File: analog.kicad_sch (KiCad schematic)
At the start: 36 parts, among them IC6 MCP6S91-E_MS, IC7 MCP6S91-E_MS, IC8 MCP4726A0T-E_CH, K1 AQY210EHAX, K2 AQY210EHAX, U10 MCP6022T-I_SN, U8 MCP6022T-I_SN, U9 MCP6022T-I_SN

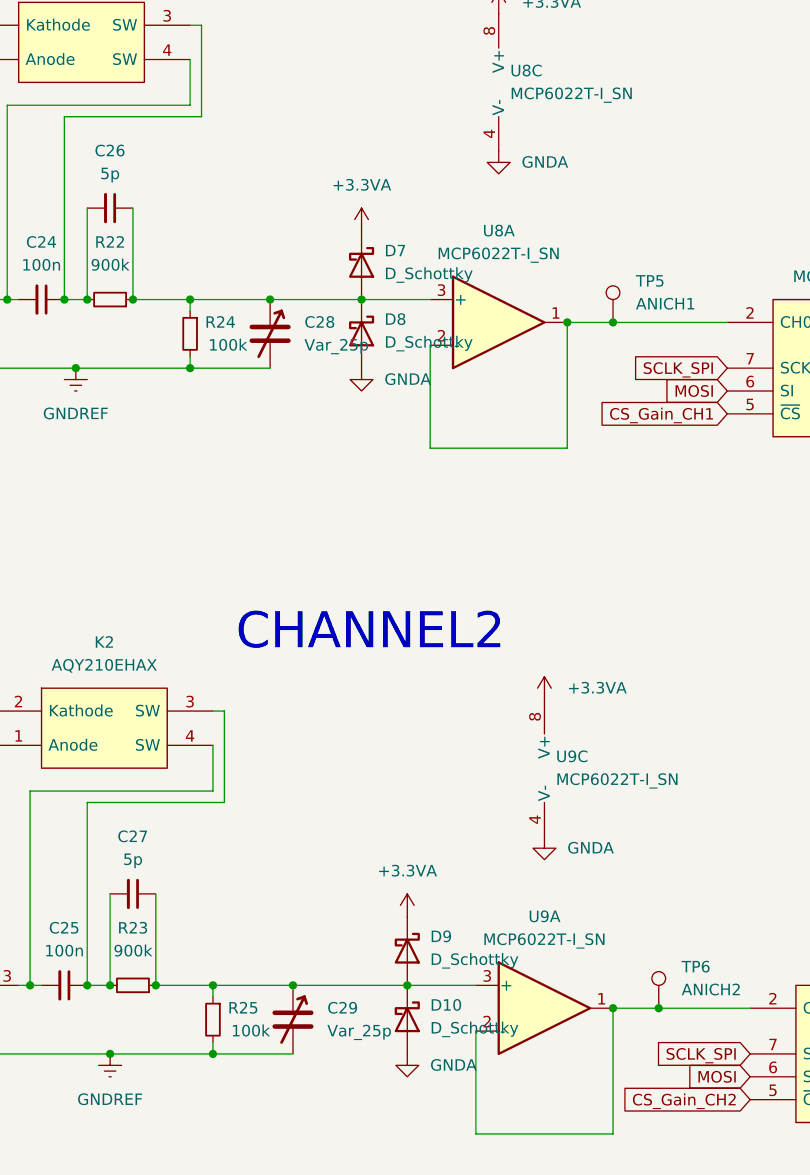
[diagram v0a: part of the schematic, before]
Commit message: last changes
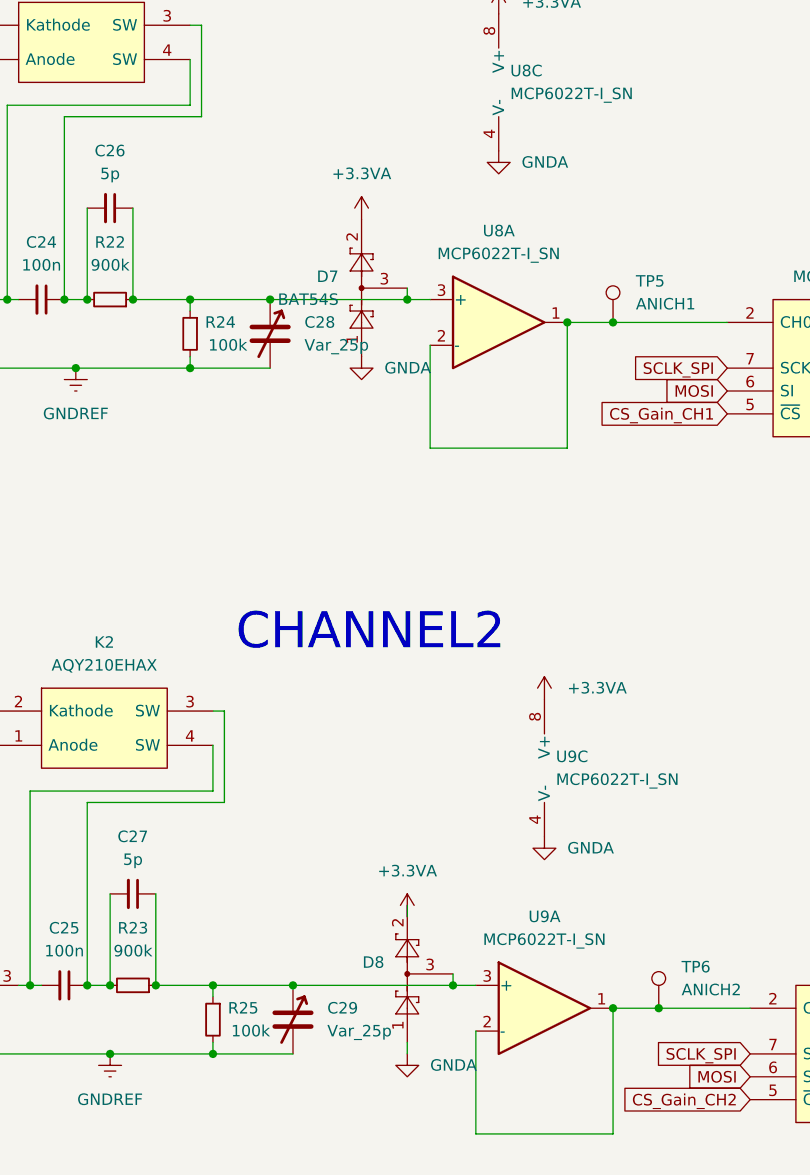
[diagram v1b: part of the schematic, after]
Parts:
- removed D10, D7, D8, D9: D_Schottky, Diode_SMD:D_0805_2012Metric_Pad1.15x1.40mm_HandSolder, symbol Device:D_Schottky
- added D7: BAT54S, Package_TO_SOT_SMD:SOT-23, symbol Diode:BAT54S
- added D8: (no value), symbol Diode:BAT54S
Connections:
- net +3.3VA: now also D7.2, D8.2
- net GNDA: now also D7.1, D8.1
- net at C27.1, C29.1, R23.1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: now also D8.3
- net at C26.1, C28.1, R22.1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: now also D7.3
